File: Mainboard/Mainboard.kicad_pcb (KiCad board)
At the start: 2 copper layers, 75 x 50 mm, 20 parts, among them J1 Conn_01x05, J2 Conn_02x08_Odd_Even, J3 Conn_02x06_Odd_Even, J4 Conn_02x06_Odd_Even, J5 Conn_02x02_Odd_Even, U1 ESP32-WROOM-32D, U2 ATxmega128A4U-AU

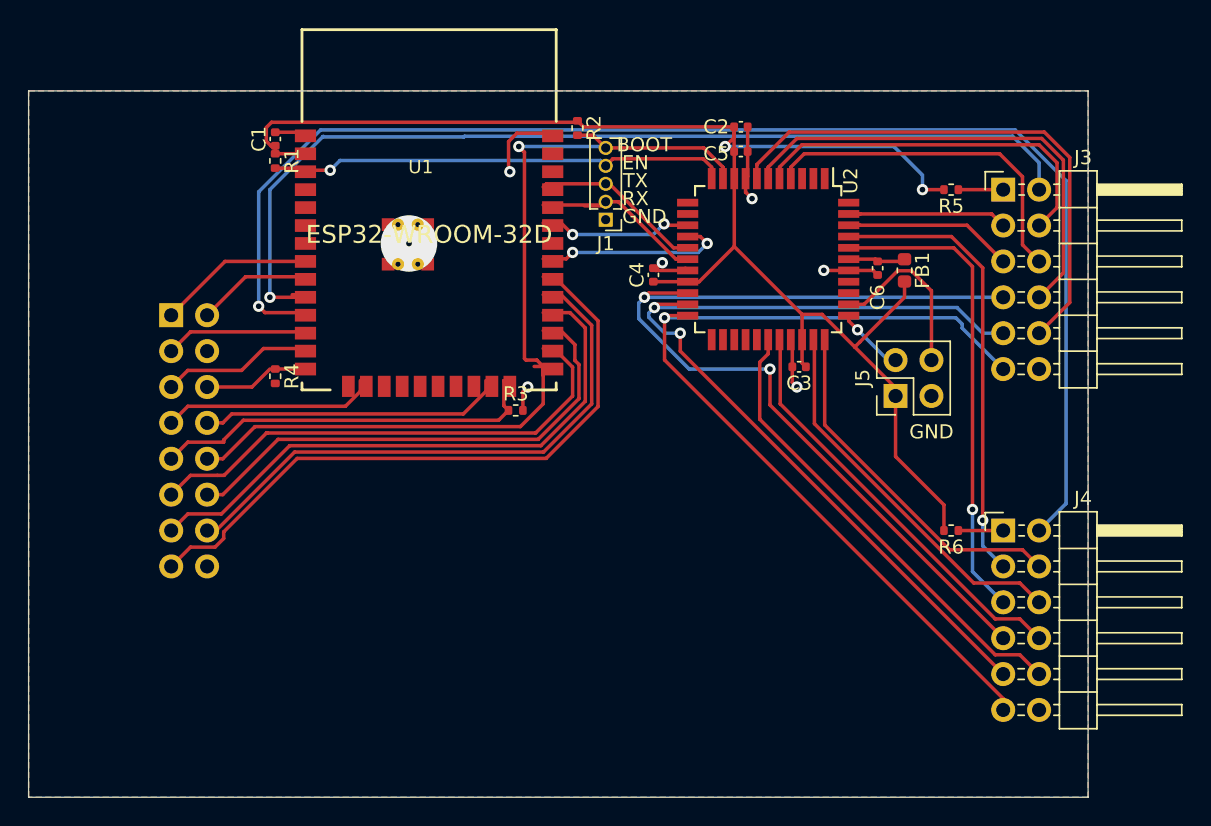
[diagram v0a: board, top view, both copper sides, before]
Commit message: Initial commit2
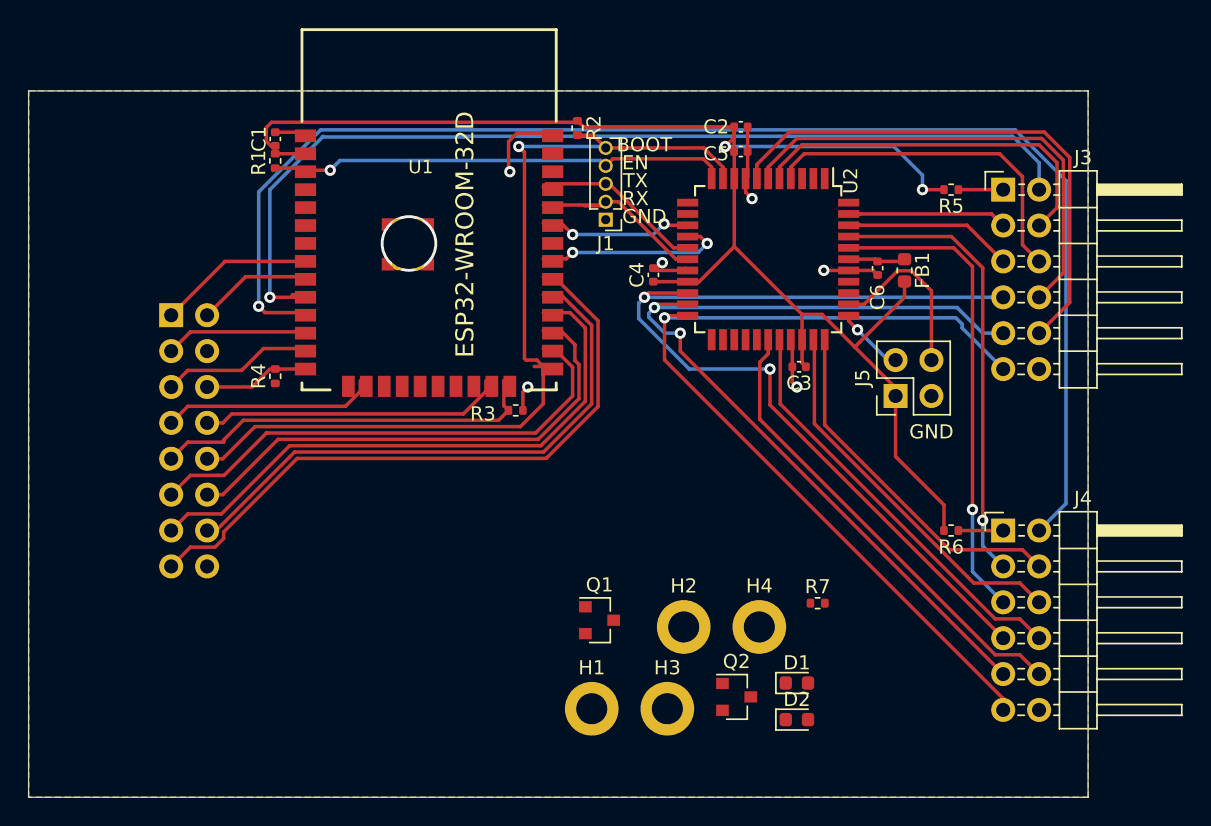
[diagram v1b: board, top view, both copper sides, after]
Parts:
- added D1: D, Diode_SMD:D_0603_1608Metric, F.Cu at (159.4, 81.9)
- added D2: D, Diode_SMD:D_0603_1608Metric, F.Cu at (159.4, 84.5)
- added H1: MountingHole_Pad, MountingHole:MountingHole_2.2mm_M2_DIN965_Pad, F.Cu at (144.9, 83.7)
- added H2: MountingHole_Pad, MountingHole:MountingHole_2.2mm_M2_DIN965_Pad, F.Cu at (151.4, 77.9)
- added H3: MountingHole_Pad, MountingHole:MountingHole_2.2mm_M2_DIN965_Pad, F.Cu at (150.2, 83.7)
- added H4: MountingHole_Pad, MountingHole:MountingHole_2.2mm_M2_DIN965_Pad, F.Cu at (156.7, 77.9)
- added Q1: BSS123, Package_TO_SOT_SMD:SOT-23, F.Cu at (145.4, 77.5)
- added Q2: AO3401A, Package_TO_SOT_SMD:SOT-23, F.Cu at (155.1, 82.9)
- added R7: 100K, Resistor_SMD:R_0402_1005Metric, F.Cu at (160.9, 76.3)
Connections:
- net GND renamed -BATT
